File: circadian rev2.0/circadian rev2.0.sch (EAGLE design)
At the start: 244 parts, among them IC1 4017D, IC10 LM4040B05, IC2 4051D, IC3 4051D, IC4 74HC595D, IC5 4053D, IC6 74HC595D, IC7 4051D, IC8 FT232RL, IC9 LM4040B10

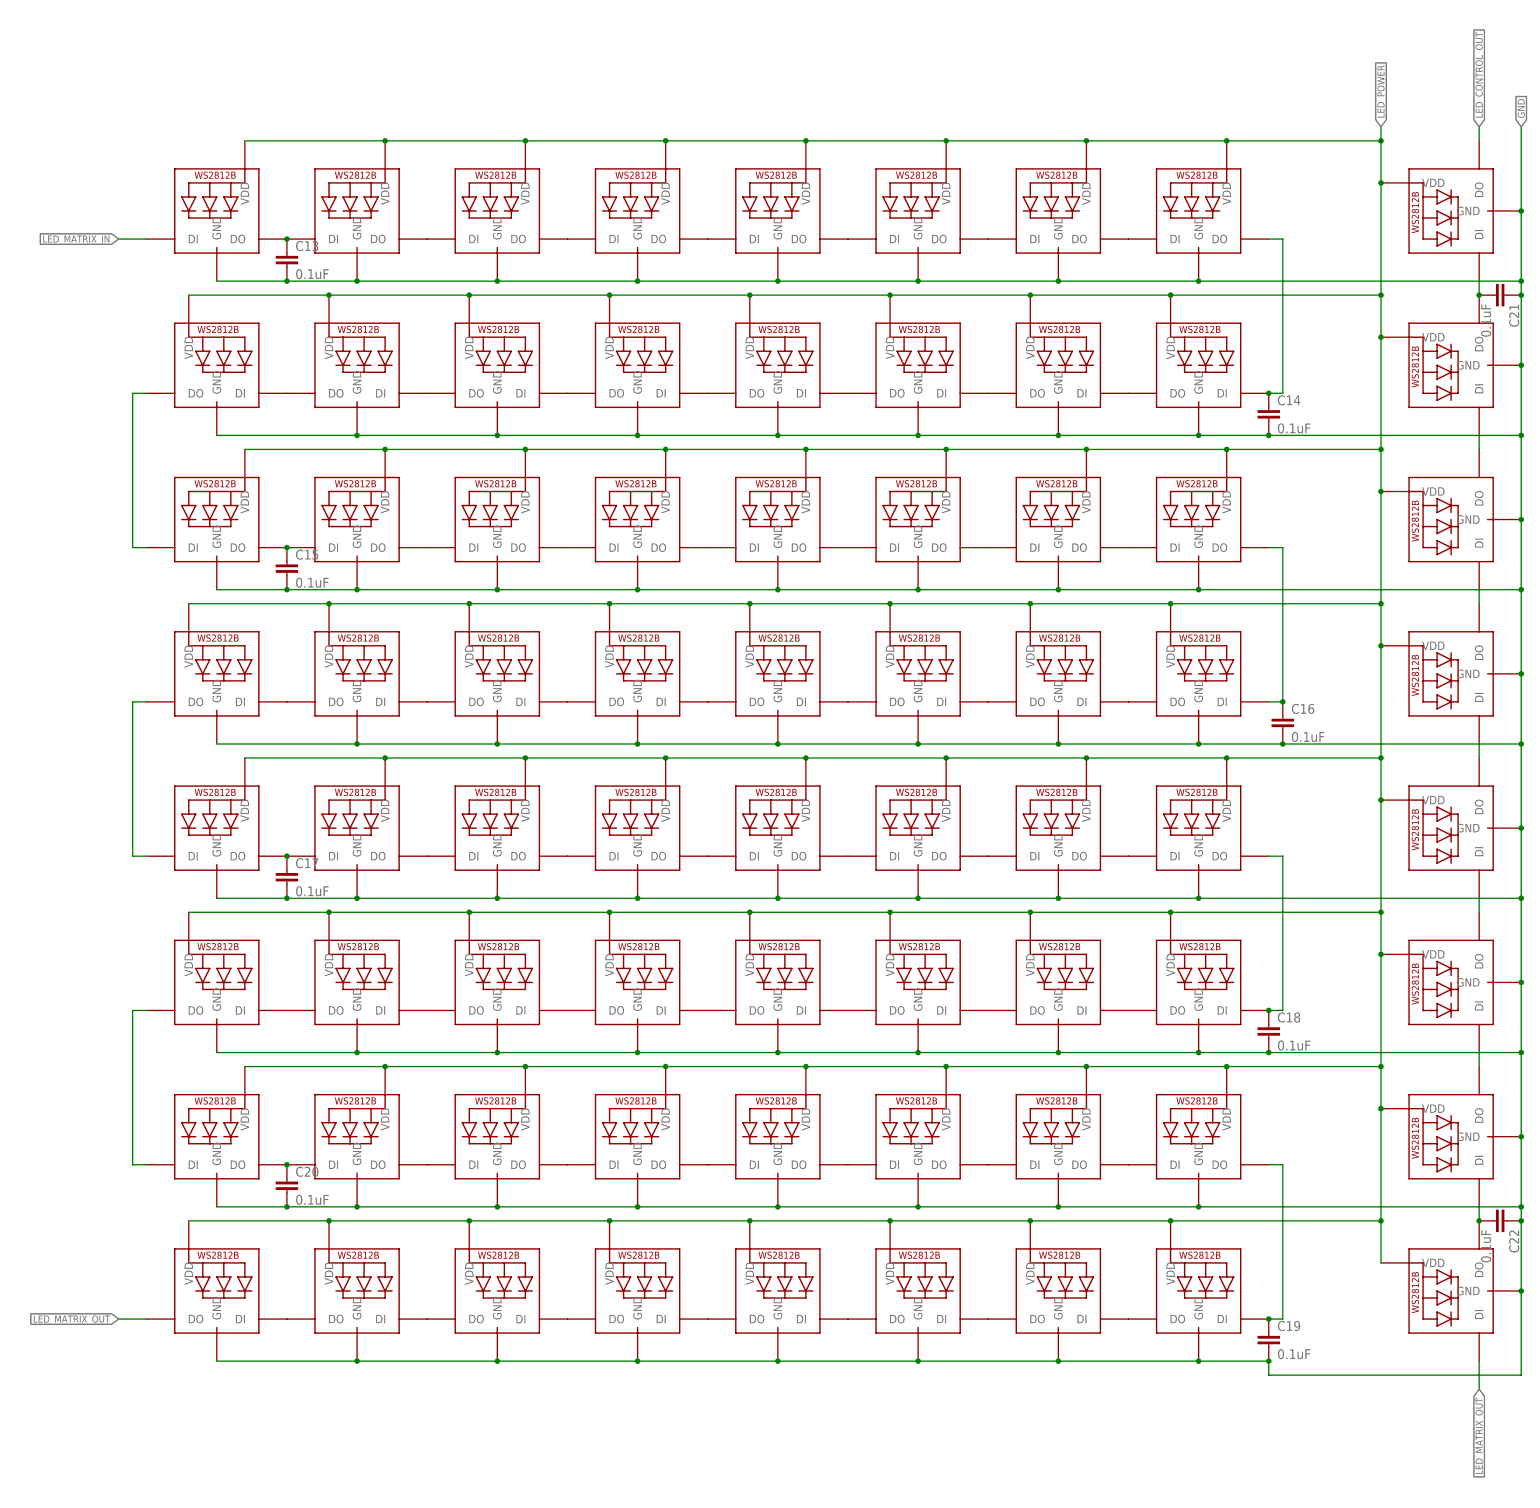
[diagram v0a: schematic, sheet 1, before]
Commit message: Add files via upload
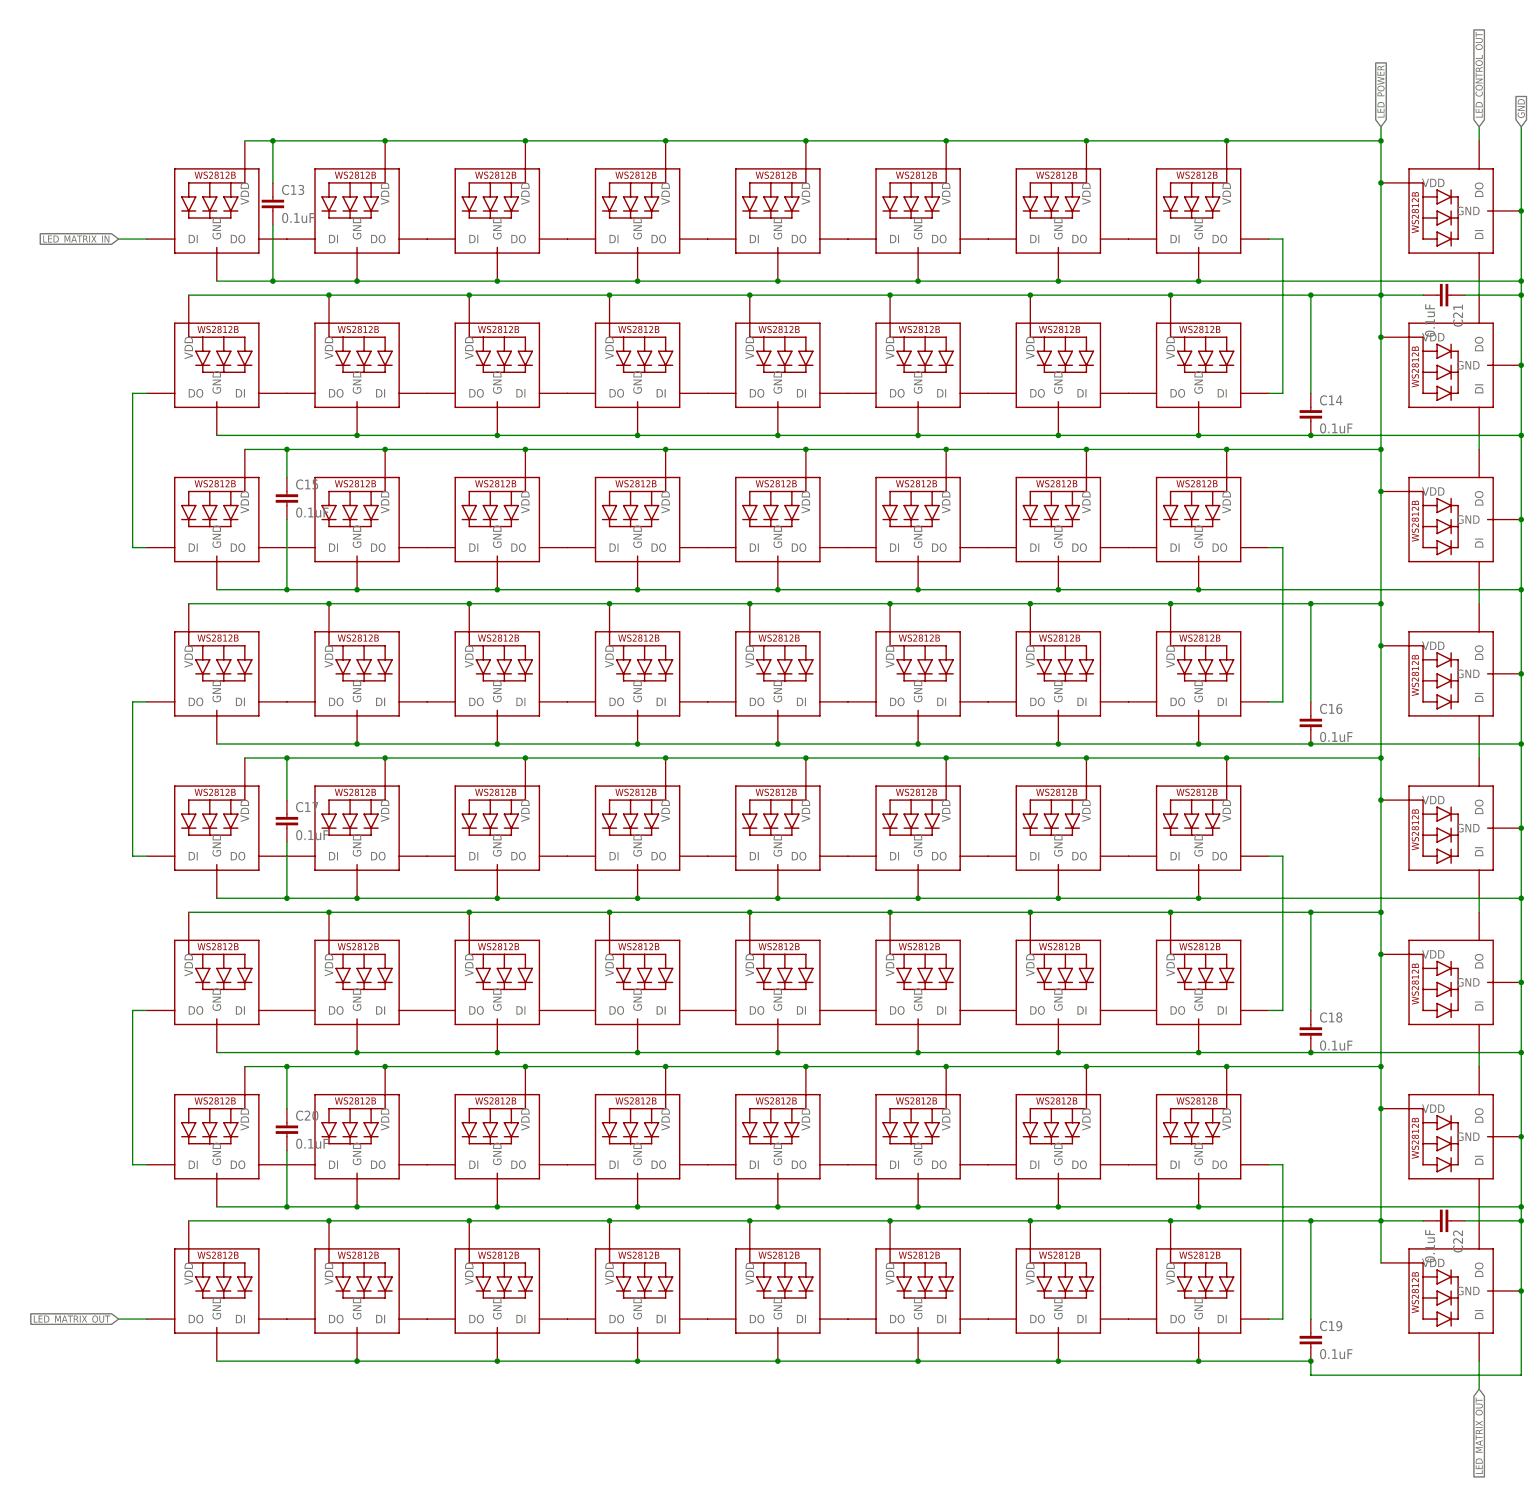
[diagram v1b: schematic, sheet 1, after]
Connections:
- removed net N$80: C21.2, LED65.DI, LED66.DO
- new net N$116: LED65.DI, LED66.DO
- net LED_POWER: now also C13.1, C14.1, C15.1, C16.1, C17.1, C18.1, C19.1, C20.1, C21.2, C22.2
- net N$12: no longer C14.1
- net N$13: no longer C15.1
- net N$22: no longer C13.1
- net N$38: no longer C16.1
- net N$39: no longer C17.1
- net N$57: no longer C18.1
- net N$58: no longer C20.1
- net N$76: no longer C19.1
- net N$86: no longer C22.2
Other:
- moved on the sheet: C13, C14, C15, C16, C17, C18, C19, C20, C21, C22
